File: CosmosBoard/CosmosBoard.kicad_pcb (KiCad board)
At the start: 4 copper layers, 200 x 100 mm, 124 parts, among them J10 Conn_01x04, J11 Conn_01x05, J12 Conn_01x25, J13 Conn_01x08, J14 Conn_01x07, J15 Conn_01x05, J16 Conn_01x04, J17 Conn_01x03, J18 Conn_01x03, J19 Conn_01x04, J2 USB_B_Micro, J20 Conn_01x02, J21 Barrel_Jack_Switch, J3 power_jumper, J4 Conn_01x25, J5 Conn_01x02, J6 Conn_01x02, J7 Conn_01x02, J8 Conn_01x02, J9 Conn_01x08, M1 Motor_Servo, M2 Motor_Servo, M3 Motor_Servo, M4 Motor_Servo, P1 SWD, SW1 SW_SPDT, SW10 SW_Push_SPDT, SW11 SW_Push_SPDT, SW2 SW_Push, SW3 SW_Push, SW4 SW_Push, SW5 SW_Push, SW6 SW_Push, SW7 RotaryEncoder_Switch, SW8 SW_Push_SPDT, SW9 SW_Push_SPDT, U1 STM32F405RGT6, U2 BNO055, U3 AMS1117-3.3, U4 BMP280, U5 E32-915T30S, U6 AMS1117-3.3, U7 AMS1117-3.3, X1 8MHz 10ppm (X50328MSB2GI), Y1 32.768, Y2 32.768

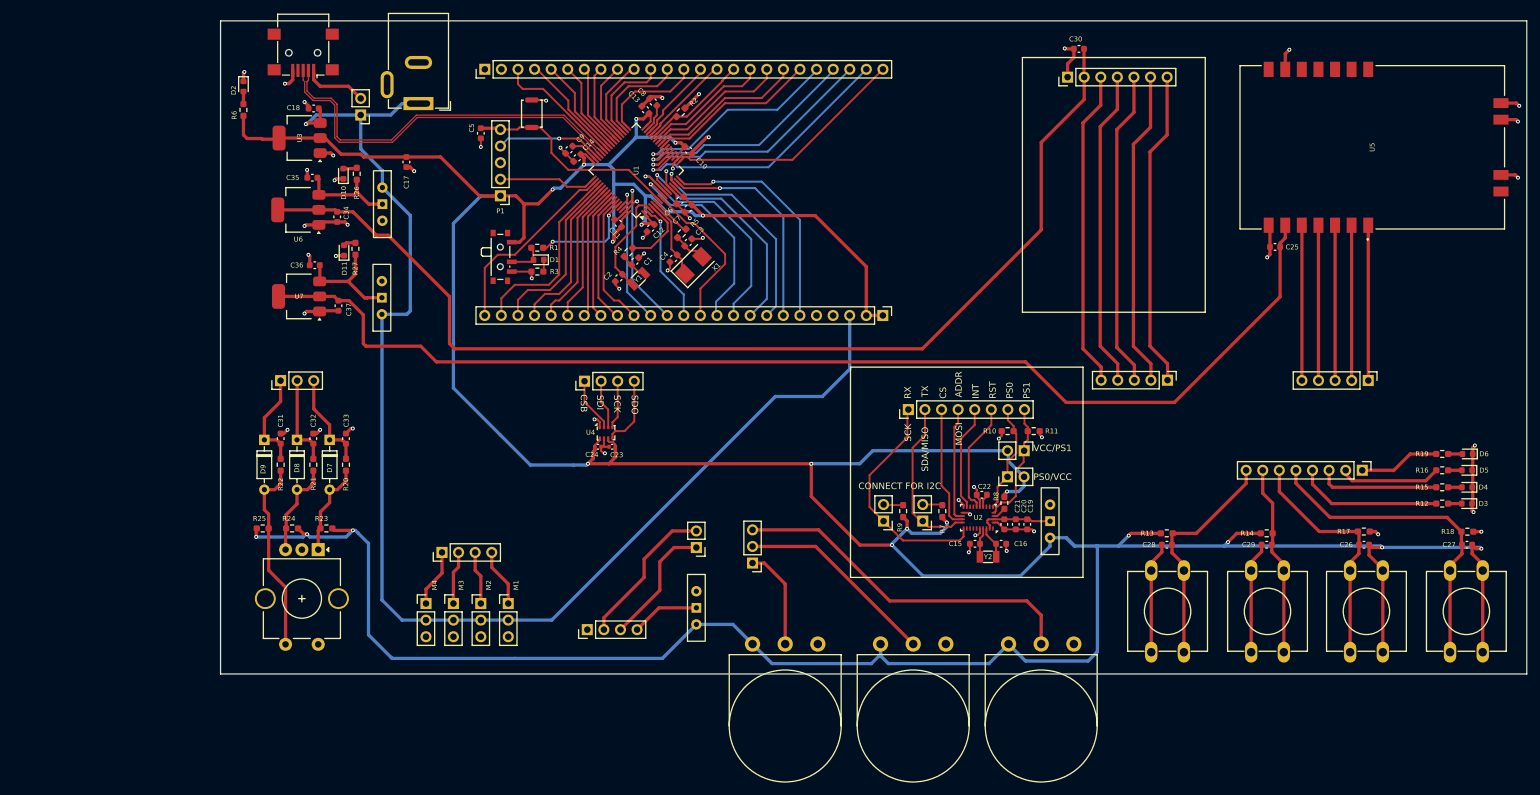
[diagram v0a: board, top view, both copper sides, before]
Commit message: pre-final
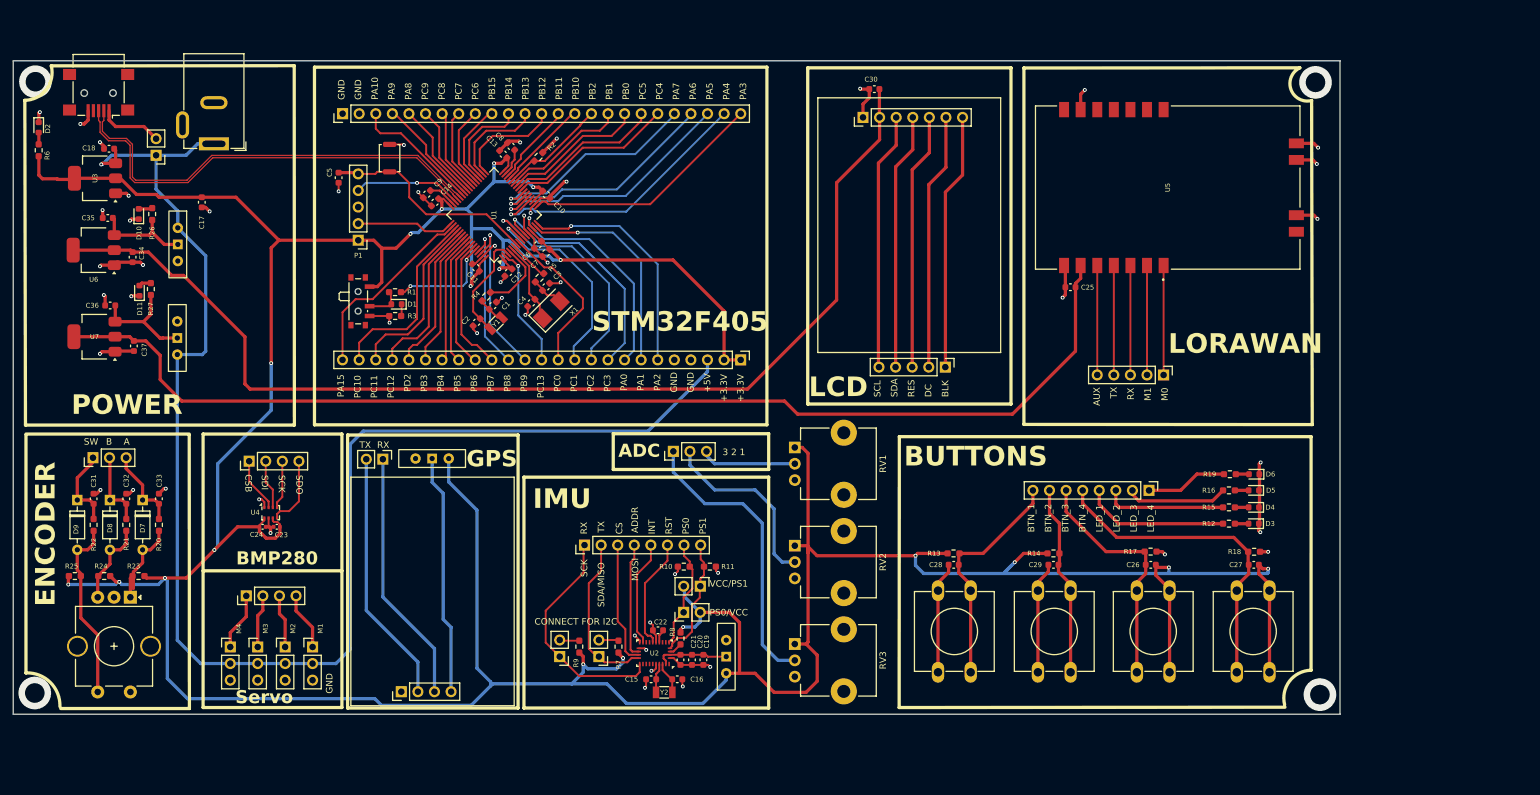
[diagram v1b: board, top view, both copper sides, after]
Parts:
- RV1, RV2, RV3: footprint Potentiometer_THT:Potentiometer_Omeg_PC16BU_Vertical -> Potentiometer_THT:Potentiometer_TT_P0915N
- moved C15 53.8 mm to (143.3, 135.0)
- moved C16 53.8 mm to (147.3, 135.0)
- moved C19 53.8 mm to (151.3, 132.0)
- moved C20 53.8 mm to (149.5, 132.0)
- moved C21 53.8 mm to (147.8, 132.0)
- moved C22 53.8 mm to (144.3, 127.5)
- moved J5 53.8 mm to (135.3, 131.5)
- moved J6 53.8 mm to (129.3, 131.5)
- moved J7 53.8 mm to (148.2, 124.8)
- moved J9 53.8 mm to (133.1, 114.4)
- moved R10 53.8 mm to (148.3, 117.8)
- moved R11 53.8 mm to (152.3, 117.8)
- moved R7 53.8 mm to (138.3, 130.0)
- moved R8 53.8 mm to (147.8, 128.7)
- moved R9 53.8 mm to (132.3, 130.0)
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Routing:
- net Net-(J17-Pin_3): track 54.0 -> 14.7 mm
- net +3V3: track 698.0 -> 668.6 mm, vias 20 -> 19
- net Net-(J17-Pin_1): track 15.5 -> 44.6 mm
- net Net-(J19-Pin_4): track 10.5 -> 36.9 mm
- net +5V: track 201.6 -> 226.0 mm
- net Net-(J19-Pin_3): track 19.4 -> 38.9 mm
- net Net-(J19-Pin_2): track 23.1 -> 38.9 mm
- net USB_D-: track 58.4 -> 68.2 mm
- net USB_D+: track 58.7 -> 68.5 mm
- net /SENSORS/SCL_disp: track 48.7 -> 39.4 mm
- net /SENSORS/RES_disp: track 48.6 -> 39.3 mm
- net /SENSORS/DC_disp: track 48.6 -> 39.3 mm
- net /SENSORS/SDA_disp: track 48.6 -> 39.3 mm
- net /SENSORS/BLK_disp: track 48.6 -> 39.3 mm
- net Net-(J11-Pin_4): track 23.8 -> 16.8 mm
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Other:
- board size 200 x 100 mm -> 203.2 x 100 mm
- board text added: "+3.3V"
- board text added: "+5V"
- board text added: "3 2 1"
- board text added: "A"
- board text added: "ADC"
- board text added: "AUX"
- board text added: "B"
- board text added: "BLK"
- board text added: "BMP280"
- board text added: "BTN_1"
- board text added: "BTN_2"
- board text added: "BTN_3"
- board text added: "BTN_4"
- board text added: "BUTTONS"
- board text added: "DC"
- board text added: "ENCODER"
- board text added: "GND"
- board text added: "GPS"
- board text added: "IMU"
- board text added: "LCD"
- board text added: "LED_1"
- board text added: "LED_2"
- board text added: "LED_3"
- board text added: "LED_4"
- board text added: "LORAWAN"
- board text added: "M0"
- board text added: "M1"
- board text added: "PA0"
- board text added: "PA1"
- board text added: "PA10"
- board text added: "PA15"
- board text added: "PA2"
- board text added: "PA3"
- board text added: "PA4"
- board text added: "PA5"
- board text added: "PA6"
- board text added: "PA7"
- board text added: "PA8"
- board text added: "PA9"
- board text added: "PB0"
- board text added: "PB1"
- board text added: "PB10"
- board text added: "PB11"
- board text added: "PB12"
- board text added: "PB13"
- board text added: "PB14"
- board text added: "PB15"
- board text added: "PB2"
- board text added: "PB3"
- board text added: "PB4"
- board text added: "PB5"
- board text added: "PB6"
- board text added: "PB7"
- board text added: "PB8"
- board text added: "PB9"
- board text added: "PC0"
- board text added: "PC1"
- board text added: "PC10"
- board text added: "PC11"
- board text added: "PC12"
- board text added: "PC13"
- board text added: "PC2"
- board text added: "PC3"
- board text added: "PC4"
- board text added: "PC5"
- board text added: "PC6"
- board text added: "PC7"
- board text added: "PC8"
- board text added: "PC9"
- board text added: "PD2"
- board text added: "POWER"
- board text added: "RES"
- board text added: "SCL"
- board text added: "SDA"
- board text added: "STM32F405"
- board text added: "SW"
- board text added: "Servo"
